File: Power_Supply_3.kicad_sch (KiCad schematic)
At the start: 14 parts

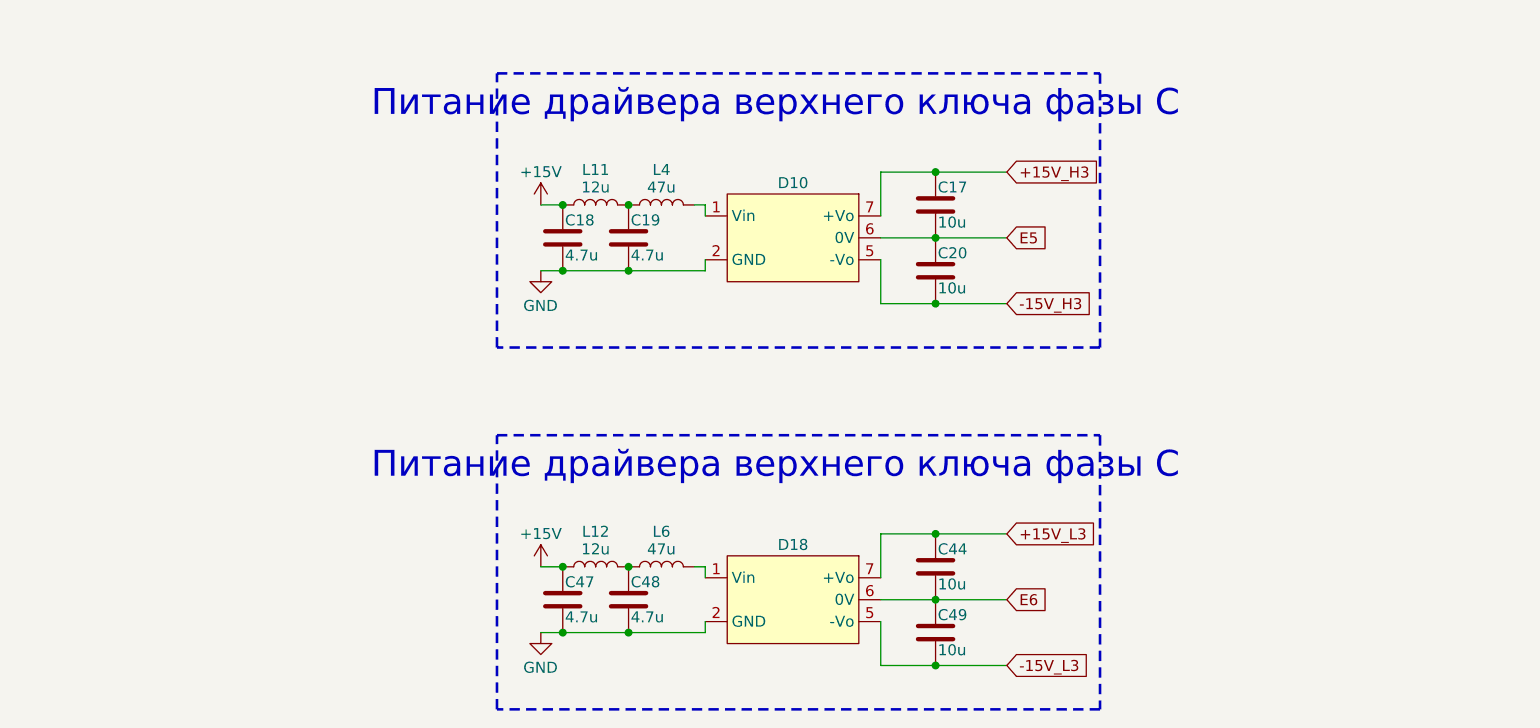
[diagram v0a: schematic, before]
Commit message: VER2.2.1: создал папку для производственных доков
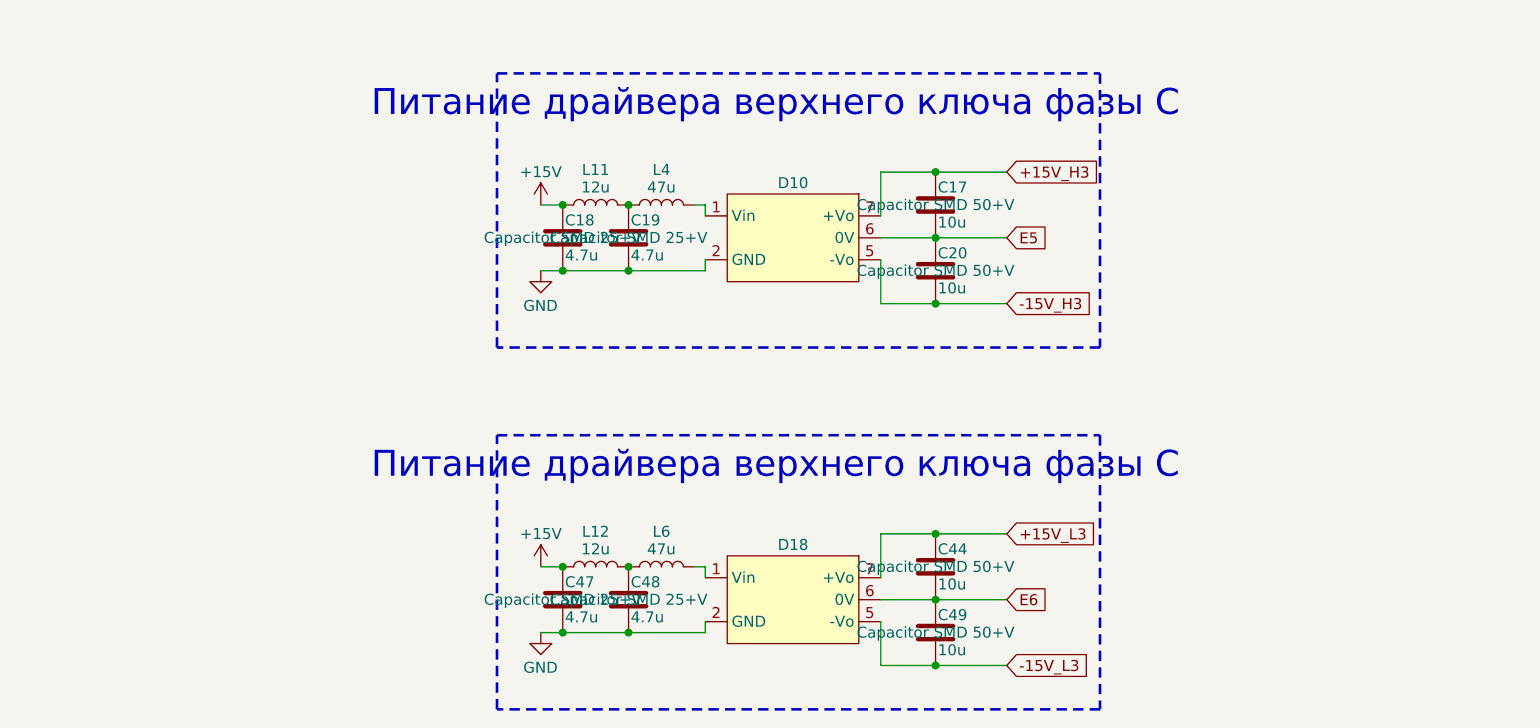
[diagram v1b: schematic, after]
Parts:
- C17, C20, C44, C49: Description P/N (none) -> Capacitor SMD 50+V
- C18, C19, C47, C48: Description P/N (none) -> Capacitor SMD 25+V
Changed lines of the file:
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@@
 			)
 		)
-		(property "Description P/N" ""
+		(property "Description P/N" "Capacitor SMD 25+V"
 			(at 129.54 91.44 0)
 			(effects
@@
 			)
 		)
-		(property "Description P/N" ""
+		(property "Description P/N" "Capacitor SMD 25+V"
 			(at 129.54 133.35 0)
 			(effects
@@
 			)
 		)
-		(property "Description P/N" ""
+		(property "Description P/N" "Capacitor SMD 25+V"
 			(at 137.16 91.44 0)
 			(effects
@@
 			)
 		)
-		(property "Description P/N" ""
+		(property "Description P/N" "Capacitor SMD 25+V"
 			(at 137.16 133.35 0)
 			(effects
@@
 			)
 		)
-		(property "Description P/N" ""
+		(property "Description P/N" "Capacitor SMD 50+V"
 			(at 172.72 87.63 0)
 			(effects
@@
 			)
 		)
-		(property "Description P/N" ""
+		(property "Description P/N" "Capacitor SMD 50+V"
 			(at 172.72 137.16 0)
 			(effects
@@
 			)
 		)
-		(property "Description P/N" ""
+		(property "Description P/N" "Capacitor SMD 50+V"
 			(at 172.72 129.54 0)
 			(effects
@@
 			)
 		)
-		(property "Description P/N" ""
+		(property "Description P/N" "Capacitor SMD 50+V"
 			(at 172.72 95.25 0)
 			(effects

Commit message: VER2.2.1: исправил все доки
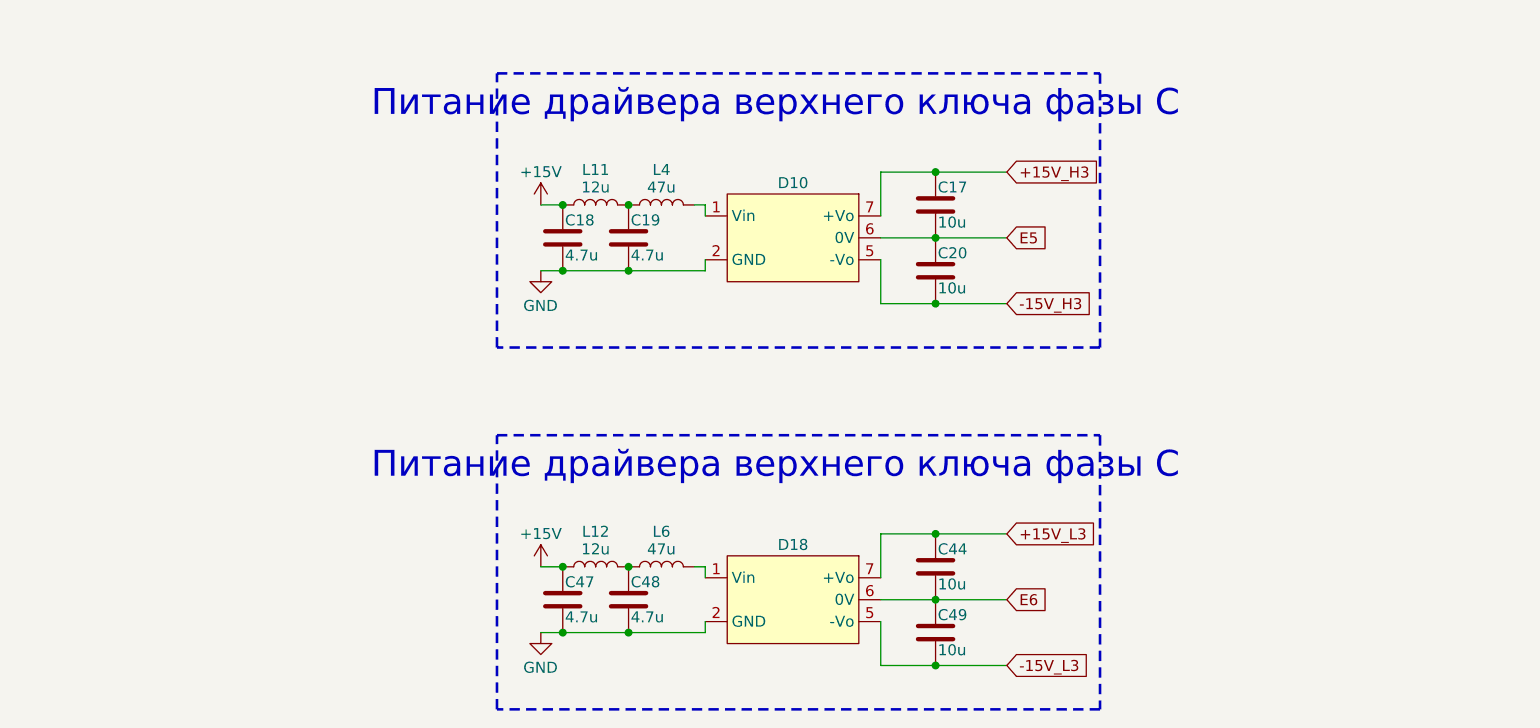
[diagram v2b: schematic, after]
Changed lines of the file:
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@@
 		(date "2025-06-04")
 		(company "ООО \"ЭТТ\"")
+		(comment 1 "НВЦТ.EVP150-2-1.2000.120_v1 Э3")
 	)
 	(rectangle
@@
 					(size 1.27 1.27)
 				)
+				(hide yes)
 			)
 		)
@@
 					(size 1.27 1.27)
 				)
+				(hide yes)
 			)
 		)
@@
 					(size 1.27 1.27)
 				)
+				(hide yes)
 			)
 		)
@@
 					(size 1.27 1.27)
 				)
+				(hide yes)
 			)
 		)
@@
 					(size 1.27 1.27)
 				)
+				(hide yes)
 			)
 		)
@@
 					(size 1.27 1.27)
 				)
+				(hide yes)
 			)
 		)
@@
 					(size 1.27 1.27)
 				)
+				(hide yes)
 			)
 		)
@@
 					(size 1.27 1.27)
 				)
-			)
-		)
+				(hide yes)
+			)
+		)

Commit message: VER2.2: исправил ошибки в доках
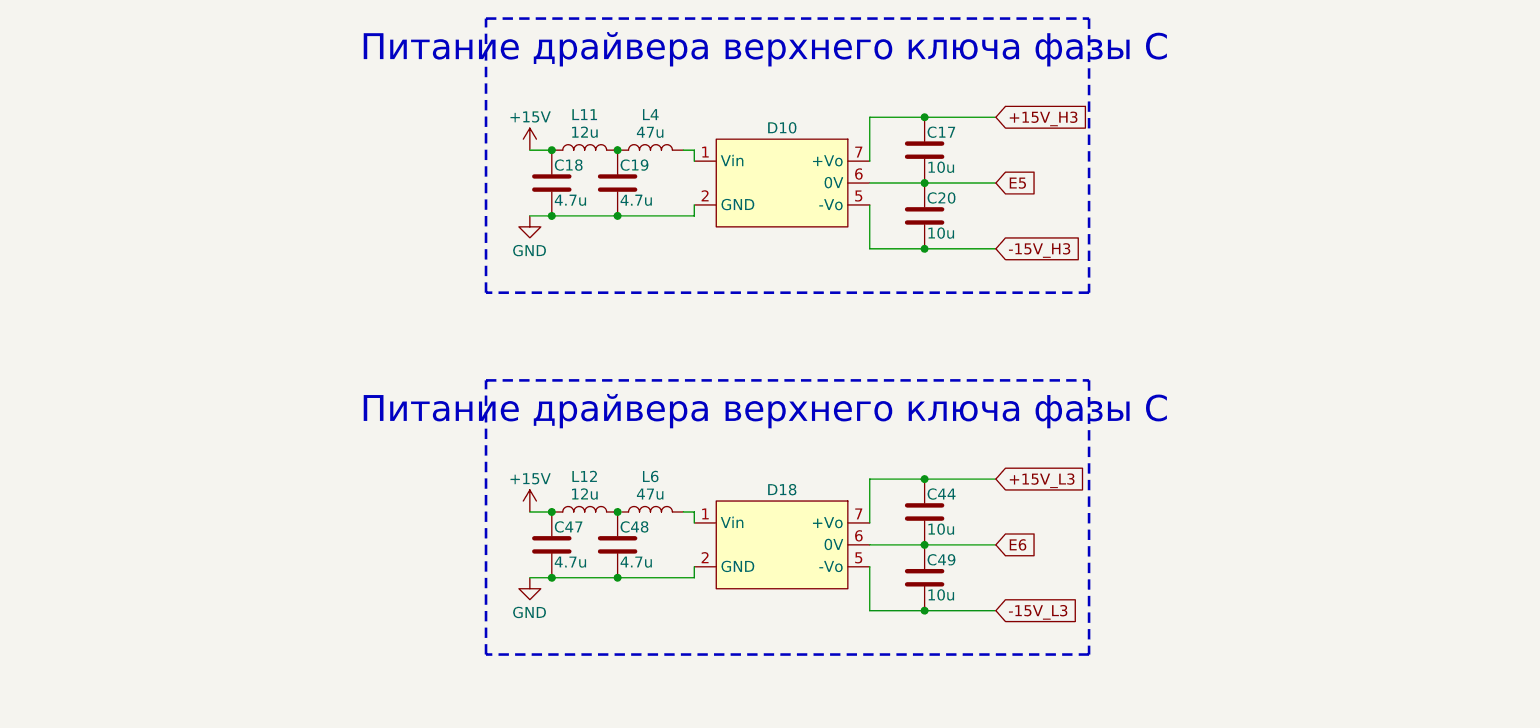
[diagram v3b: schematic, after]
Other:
- moved on the sheet: C17, C18, C19, C20, C44, C47, C48, C49, D10, D18, L11, L12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
